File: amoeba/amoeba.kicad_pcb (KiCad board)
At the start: 2 copper layers, 18.8 x 16.1 mm, 17 parts

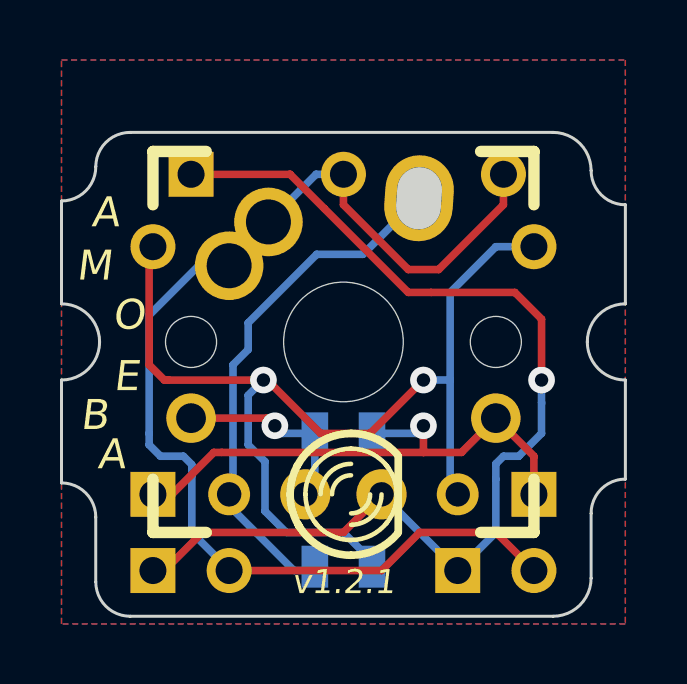
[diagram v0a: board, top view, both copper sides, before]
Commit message: Minor clean-up.
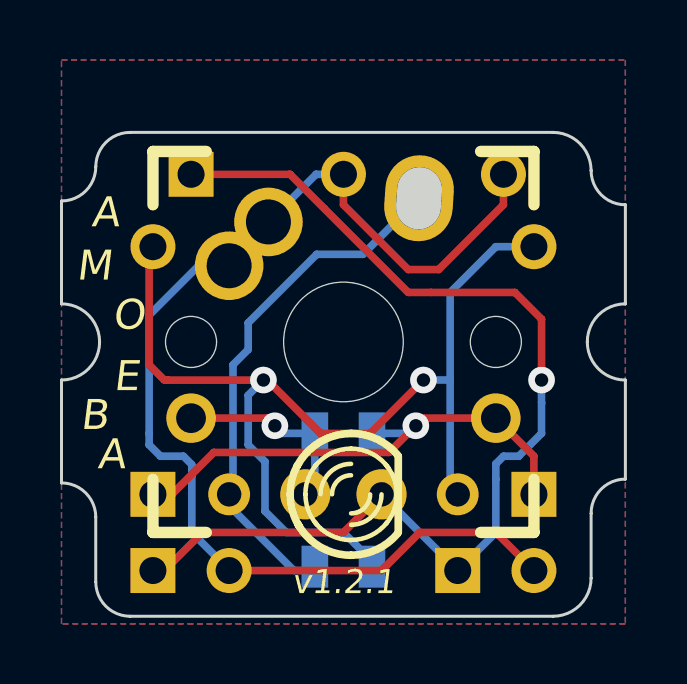
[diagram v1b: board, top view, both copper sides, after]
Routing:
- net /key/LR0: track 18.6 -> 17.1 mm
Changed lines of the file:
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@@
     (thickness 1.6)
     (drawings 68)
-    (tracks 103)
+    (tracks 99)
     (zones 0)
     (modules 17)
@@
     (18 B.Paste user hide)
     (19 F.Paste user hide)
-    (20 B.SilkS user)
+    (20 B.SilkS user hide)
     (21 F.SilkS user hide)
     (22 B.Mask user hide)
@@
     (pad_to_mask_clearance 0)
     (aux_axis_origin 0 0)
-    (visible_elements FFFFB23F)
+    (visible_elements FFFFFB3F)
     (pcbplotparams
       (layerselection 284196865)
@@
   (segment (start 244.221 116.84) (end 248.92 116.84) (width 0.254) (layer F.Cu) (net 1))
   (segment (start 242.951 118.11) (end 244.221 116.84) (width 0.254) (layer F.Cu) (net 1))
-  (segment (start 249.8725 113.538) (end 251.333 113.538) (width 0.254) (layer B.Cu) (net 2))
-  (via (at 251.587 113.284) (size 0.889) (layers F.Cu B.Cu) (net 2))
-  (segment (start 251.587 113.284) (end 251.587 114.173) (width 0.254) (layer F.Cu) (net 2))
-  (segment (start 251.333 113.538) (end 251.587 113.284) (width 0.254) (layer B.Cu) (net 2))
+  (segment (start 244.602 114.173) (end 250.444 114.173) (width 0.254) (layer F.Cu) (net 2))
+  (segment (start 243.205 115.57) (end 244.602 114.173) (width 0.254) (layer F.Cu) (net 2))
+  (segment (start 242.57 115.57) (end 243.205 115.57) (width 0.254) (layer F.Cu) (net 2))
+  (segment (start 250.444 114.173) (end 251.333 113.284) (width 0.254) (layer F.Cu) (net 2))
+  (segment (start 254 113.03) (end 251.587 113.03) (width 0.254) (layer F.Cu) (net 2) (status 400000))
+  (segment (start 251.587 113.03) (end 251.333 113.284) (width 0.254) (layer F.Cu) (net 2))
+  (segment (start 249.8725 113.538) (end 251.079 113.538) (width 0.254) (layer B.Cu) (net 2) (status 400000))
+  (segment (start 251.079 113.538) (end 251.333 113.284) (width 0.254) (layer B.Cu) (net 2))
+  (via (at 251.333 113.284) (size 0.889) (layers F.Cu B.Cu) (net 2))
   (segment (start 255.27 115.57) (end 255.27 114.3) (width 0.254) (layer F.Cu) (net 2))
   (segment (start 255.27 114.3) (end 254 113.03) (width 0.254) (layer F.Cu) (net 2))
-  (segment (start 242.57 115.57) (end 243.205 115.57) (width 0.254) (layer F.Cu) (net 2))
-  (segment (start 243.205 115.57) (end 244.602 114.173) (width 0.254) (layer F.Cu) (net 2))
-  (segment (start 244.602 114.173) (end 244.856 114.173) (width 0.254) (layer F.Cu) (net 2))
-  (segment (start 244.856 114.173) (end 251.587 114.173) (width 0.254) (layer F.Cu) (net 2))
-  (segment (start 251.587 114.173) (end 252.857 114.173) (width 0.254) (layer F.Cu) (net 2))
-  (segment (start 252.857 114.173) (end 254 113.03) (width 0.254) (layer F.Cu) (net 2))
-  (segment (start 253.746 113.284) (end 254 113.03) (width 0.254) (layer F.Cu) (net 2))
   (segment (start 243.8654 114.9604) (end 243.8654 114.5794) (width 0.254) (layer B.Cu) (net 3))
   (segment (start 245.11 118.0846) (end 243.8654 116.84) (width 0.254) (layer B.Cu) (net 3))
@@
   (segment (start 242.443 113.538) (end 242.443 109.982) (width 0.254) (layer B.Cu) (net 3))
   (segment (start 245.11 107.95) (end 244.094 107.95) (width 0.254) (layer B.Cu) (net 3))
-  (segment (start 245.11 118.0846) (end 245.11 118.11) (width 0.254) (layer B.Cu) (net 3))
   (segment (start 242.443 113.919) (end 242.443 113.538) (width 0.254) (layer B.Cu) (net 3))
   (segment (start 242.824 114.3) (end 242.443 113.919) (width 0.254) (layer B.Cu) (net 3))
@@
   (segment (start 246.3038 114.4778) (end 245.745 113.919) (width 0.254) (layer B.Cu) (net 4))
   (segment (start 246.3038 116.1288) (end 246.3038 114.4778) (width 0.254) (layer B.Cu) (net 4))
-  (segment (start 251.587 111.76) (end 251.587 112.014) (width 0.254) (layer F.Cu) (net 4))
   (via (at 251.587 111.76) (size 0.889) (layers F.Cu B.Cu) (net 4))
   (segment (start 251.587 111.76) (end 252.476 111.76) (width 0.254) (layer B.Cu) (net 4))
